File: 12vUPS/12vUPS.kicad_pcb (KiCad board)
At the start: 2 copper layers, 79 x 61 mm, 20 parts, among them J1 INPUT, J2 BATTERY, J3 OUTPUT, J4 ENABLE, K1 VEGHA L08A0212VDC, K2 VEGHA L08A0212VDC, Q1 BDX53C

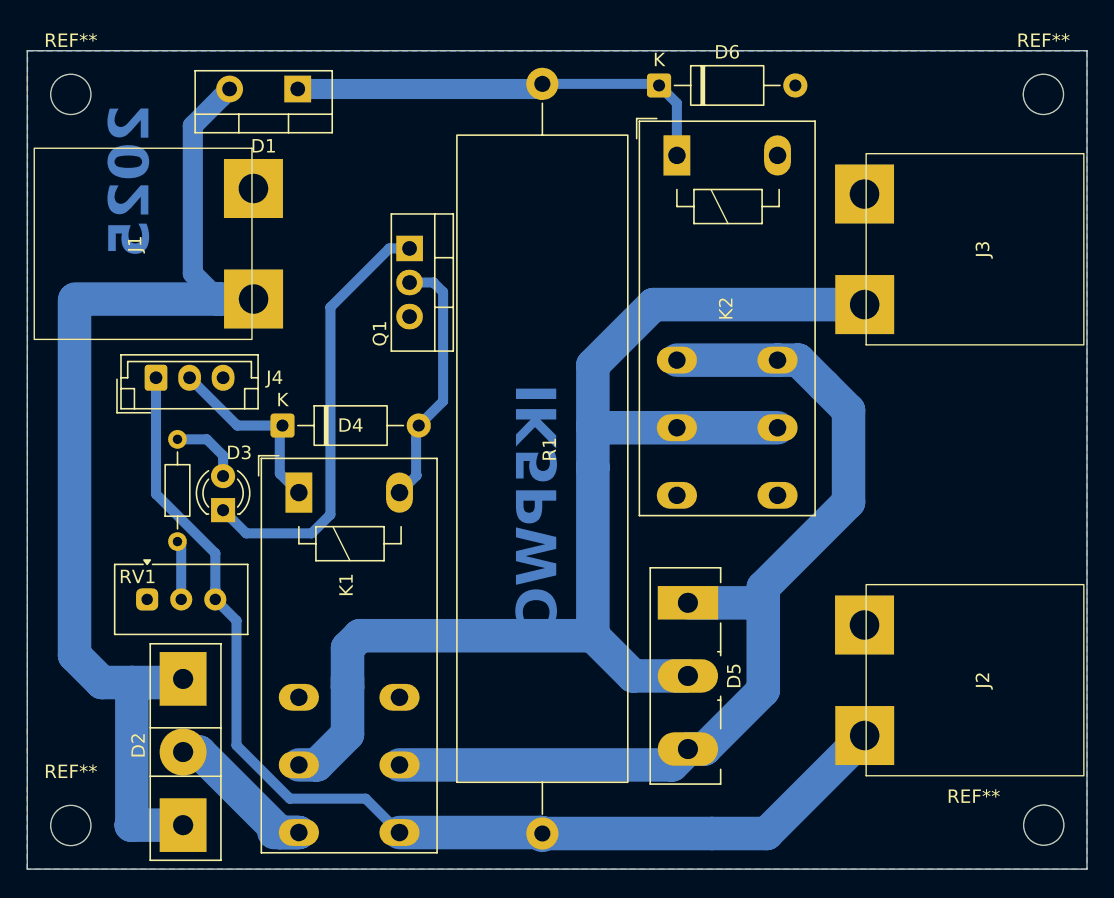
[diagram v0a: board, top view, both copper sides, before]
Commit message: Update 12vUPS-2025-06-10_185612.zip, 12vUPS-2025-06-10_190121.zip, 12vUPS-2025-06-10_190645.zip, and 3 more files
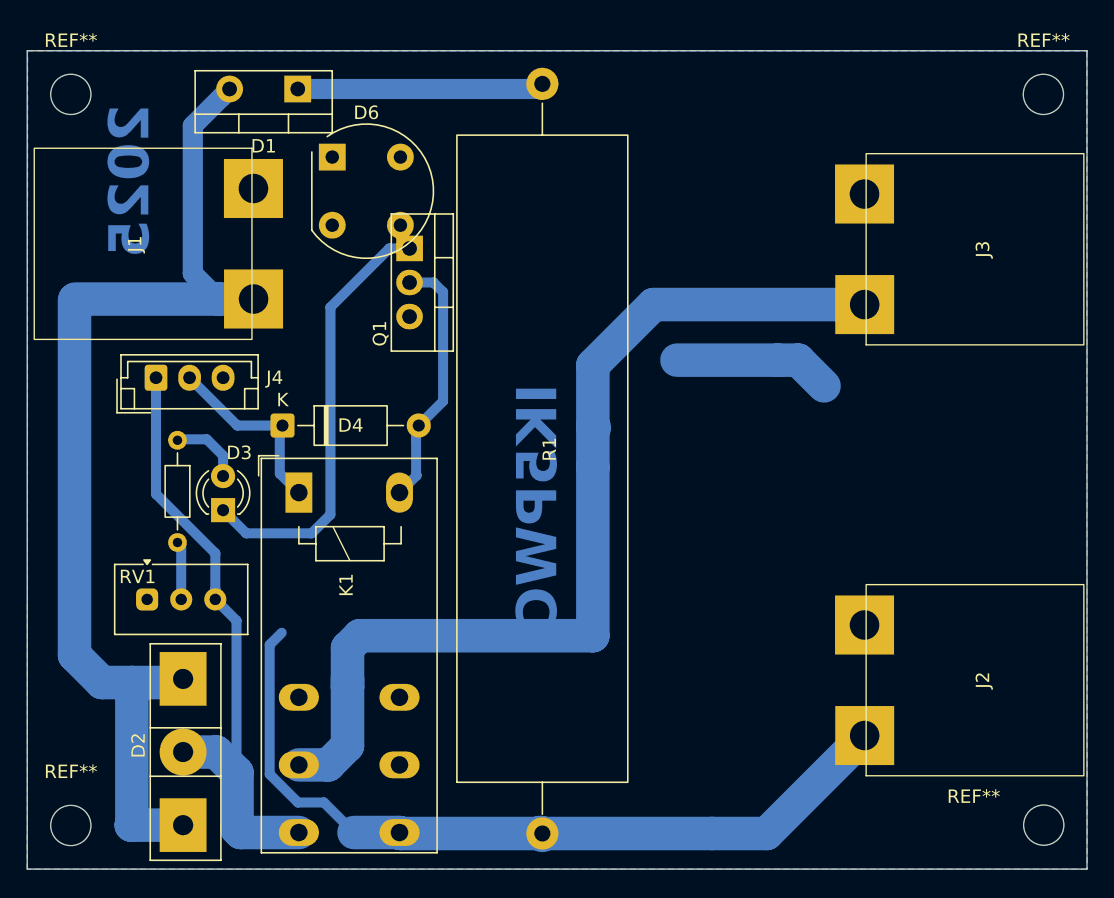
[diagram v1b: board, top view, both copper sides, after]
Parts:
- removed D5: D_Schottky_Dual_CommonCathode_AKA_Parallel, Package_TO_SOT_THT:TO-247-3_Vertical
- removed K2: VEGHA L08A0212VDC, IK5PWC:VEGhA L08 12V dc
- D6: value 1N4001 -> W01G; footprint Diode_THT:D_A-405_P10.16mm_Horizontal -> Diode_THT:Diode_Bridge_Round_D9.8mm
- moved D6 24.9 mm to (35.5, 24.3)
- moved R2 7.55 mm to (24.0, 45.4), turned to -90 degrees
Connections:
- D1 pad 1: /X1 -> Net-(D1-K)
- D1 pad 2: VCC -> /INPUT
- D2 pad 2: VCC -> /INPUT
- D6 pad 1: /X1 -> Net-(D6-+)
- D6 pad 2: GND -> /OUT
- J1 pad 2: VCC -> /INPUT
- J2 pad 1: /+12V -> /BATT
- J3 pad 1: Net-(D5-K) -> /OUT
- J4 pad 1: /+12V -> /BATT
- K1 pad 11: Net-(D5-K) -> /OUT
- K1 pad 24: /+12V -> /BATT
- R1 pad 1: /+12V -> /BATT
- R1 pad 2: /X1 -> Net-(D1-K)
- R2 pad 1: Net-(R2-Pad1) -> Net-(D3-A)
- R2 pad 2: Net-(D3-A) -> Net-(R2-Pad2)
- RV1 pad 2: Net-(R2-Pad1) -> Net-(R2-Pad2)
- RV1 pad 3: /+12V -> Net-(D6-+)
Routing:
- net Net-(D5-K): track 94.8 -> 0.00 mm
- net /OUT: track 0.00 -> 85.1 mm
- net /+12V: track 82.8 -> 0.00 mm
- net VCC: track 78.2 -> 0.00 mm
- net /INPUT: track 0.00 -> 78.2 mm
- net Net-(D7-A): track 72.9 -> 0.00 mm
- net /BATT: track 0.00 -> 60.5 mm
- net /X1: track 33.6 -> 0.00 mm
- net Net-(D2-K): track 13.0 -> 45.5 mm
- net Net-(D1-K): track 0.00 -> 19.1 mm
- net Net-(R2-Pad2): track 0.00 -> 4.43 mm
- net Net-(R2-Pad1): track 4.43 -> 0.00 mm

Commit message: Update #auto_saved_files#, 12vUPS-2025-06-02_175555.zip, 12vUPS-2025-06-02_180136.zip, and 18 more files
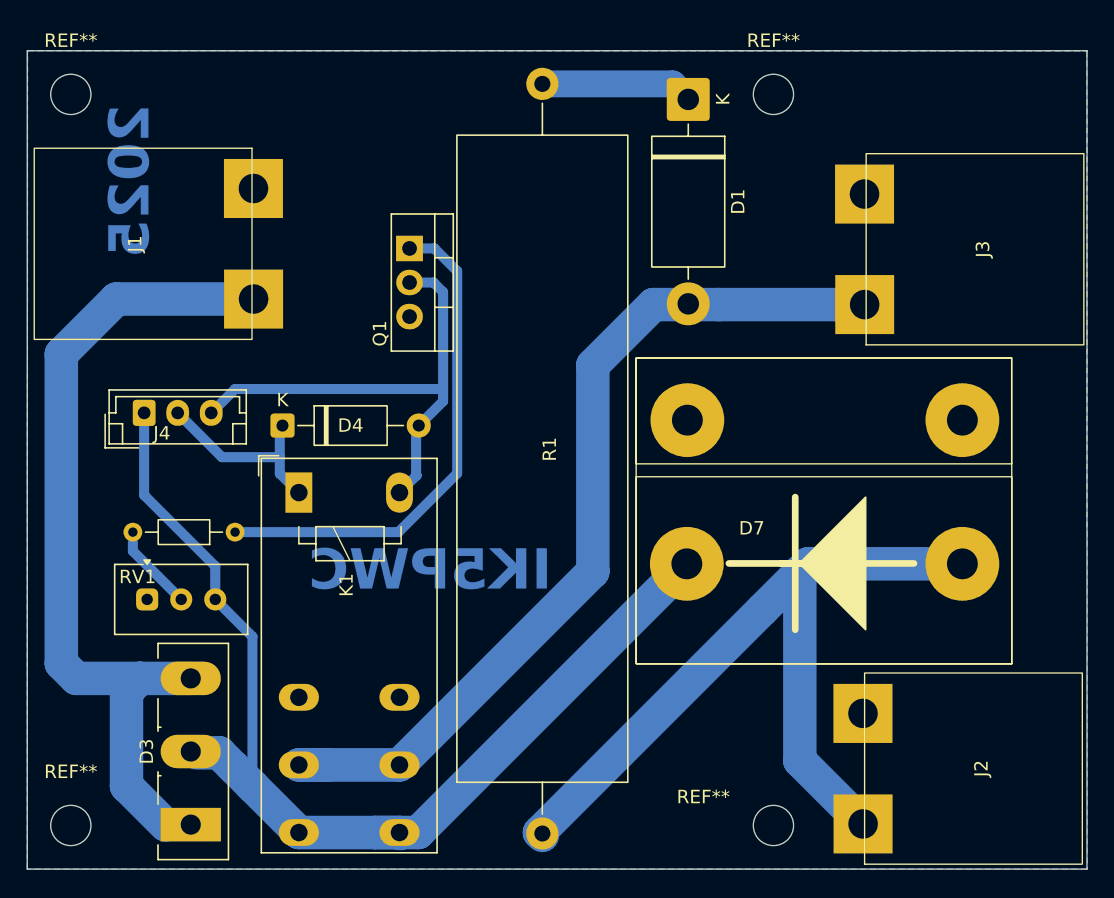
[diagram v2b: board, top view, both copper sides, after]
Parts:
- removed D2: 30CPF04, IK5PWC:30CPF04
- removed D6: W01G, Diode_THT:Diode_Bridge_Round_D9.8mm
- added D7: D_Ideal, IK5PWC:D_IDEAL_with_GND, F.Cu at (76.3, 58.9)
- D1: value BYW19 -> SF30GG; footprint Package_TO_SOT_THT:TO-220-2_Vertical -> Diode_THT:D_DO-201AD_P15.24mm_Horizontal
- D3: value LED_Small -> 60CPQ150; footprint LED_THT:LED_D3.0mm -> Package_TO_SOT_THT:TO-247-3_Vertical
- moved D1 29.1 mm to (62.1, 20.0), turned to -90 degrees
- moved D3 23.6 mm to (25.0, 74.1)
- moved REF** 20.1 mm to (68.4, 74.1)
- moved REF** 20.1 mm to (68.4, 19.6)
- moved R2 8.08 mm to (28.3, 52.3), turned to 180 degrees
- moved J2 6.59 mm to (75.1, 74.0)
- moved J4 2.76 mm to (21.5, 43.4)
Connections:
- D1 pad 2: /INPUT -> /OUT
- D3 pad 1: Net-(D3-K) -> /DC_IN
- D3 pad 2: Net-(D3-A) -> /DC-IN-RELE
- D4 pad 2: Net-(D4-A) -> /BJT-GND
- J1 pad 2: /INPUT -> /DC_IN
- J2 pad 1: /BATT -> /BATT_IN
- J4 pad 1: /BATT -> /DC-IN-RELE
- J4 pad 3: GND -> /BJT-GND
- K1 pad 14: Net-(D2-K) -> /DC-IN-RELE
- K1 pad 21: Net-(D7-A) -> /OUT
- K1 pad 24: /BATT -> /DC-IN-RELE
- K1 pad A2: Net-(D4-A) -> /BJT-GND
- Q1 pad 1: Net-(D3-K) -> Net-(Q1-B)
- Q1 pad 2: Net-(D4-A) -> /BJT-GND
- R1 pad 1: /BATT -> /BATT_IN
- R2 pad 1: Net-(D3-A) -> Net-(Q1-B)
- RV1 pad 3: Net-(D6-+) -> /DC-IN-RELE
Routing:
- net /DC-IN-RELE: track 0.00 -> 80.4 mm
- net /INPUT: track 78.2 -> 0.00 mm
- net /BATT_IN: track 0.00 -> 62.0 mm
- net /DC_IN: track 0.00 -> 61.8 mm
- net /BATT: track 60.5 -> 0.00 mm
- net Net-(D2-K): track 45.5 -> 0.00 mm
- net Net-(Q1-B): track 0.00 -> 37.7 mm
- net /BJT-GND: track 0.00 -> 37.5 mm
- net Net-(D3-K): track 32.5 -> 0.00 mm
- net Net-(D4-A): track 19.3 -> 0.00 mm
- net /OUT: track 85.1 -> 67.6 mm
- net Net-(D1-K): track 19.1 -> 12.2 mm
- net Net-(D3-A): track 5.43 -> 0.00 mm
- net Net-(R2-Pad2): track 4.43 -> 5.75 mm
- net /ENA: track 14.0 -> 14.5 mm

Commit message: Update 12vUPS-2025-06-06_224542.zip, 12vUPS-2025-06-06_225111.zip, 12vUPS-2025-06-06_225614.zip, and 28 more files
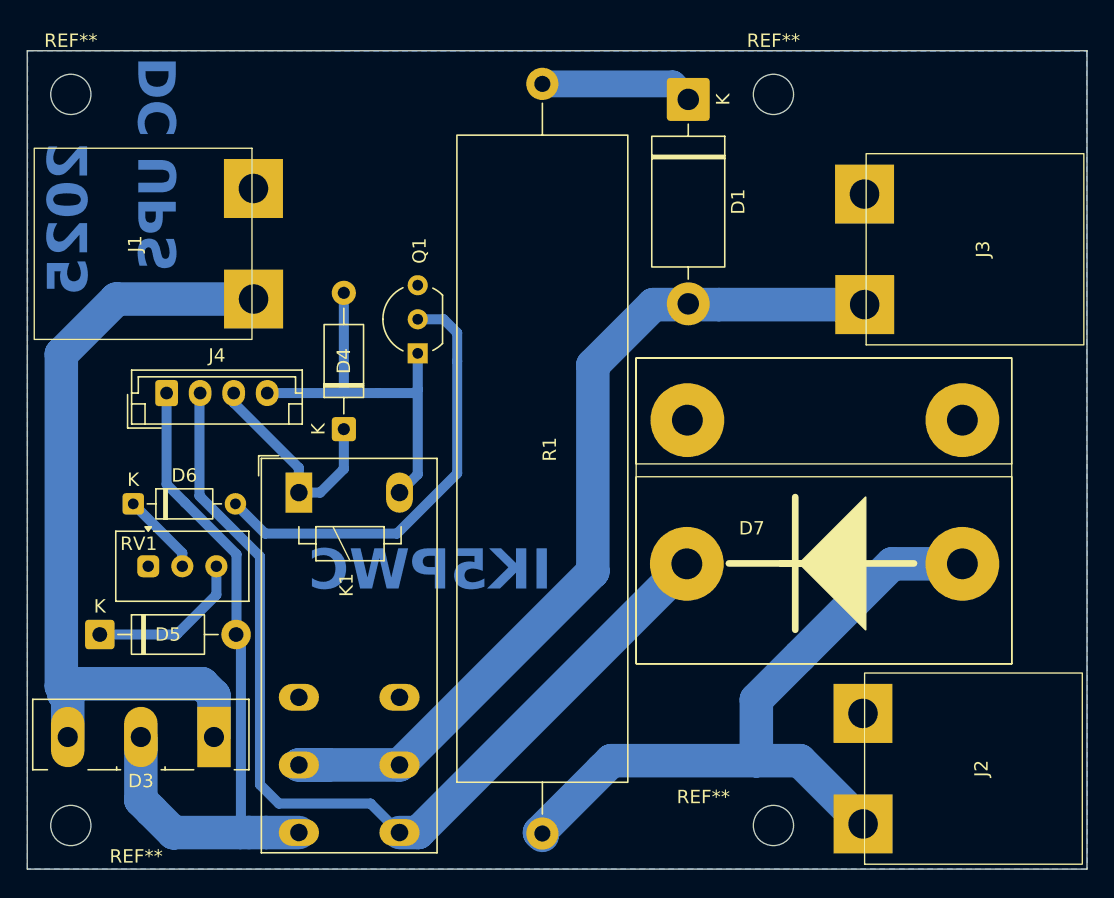
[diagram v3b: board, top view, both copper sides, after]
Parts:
- removed R2: 510, Resistor_THT:R_Axial_DIN0204_L3.6mm_D1.6mm_P7.62mm_Horizontal
- added D5: D, Diode_THT:D_DO-41_SOD81_P10.16mm_Horizontal, F.Cu at (18.2, 59.9)
- added D6: 4V1, Diode_THT:D_DO-35_SOD27_P7.62mm_Horizontal, F.Cu at (20.7, 50.2)
- J4: footprint Connector_JST:JST_EH_B3B-EH-A_1x03_P2.50mm_Vertical -> Connector_JST:JST_EH_B4B-EH-A_1x04_P2.50mm_Vertical
- Q1: value BDX53C -> BC337; footprint Package_TO_SOT_THT:TO-220-3_Vertical -> Package_TO_SOT_THT:TO-92_Inline_Wide
- moved Q1 7.84 mm to (41.9, 38.9), turned to 90 degrees
- moved D3 6.76 mm to (26.7, 67.5), turned to 180 degrees
- moved D4 4.58 mm to (36.4, 44.6), turned to 90 degrees
- moved RV1 2.47 mm to (21.8, 54.8)
- moved J4 2.23 mm to (23.2, 41.9)
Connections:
- D7 pad 1: /DC-IN-RELE -> Net-(D7-K)
- J4 pad 2: /ENA -> Net-(D7-K)
- J4 pad 3: /BJT-GND -> /ENA
- K1 pad 24: /DC-IN-RELE -> Net-(D7-K)
- Q1 pad 1: Net-(Q1-B) -> /BJT-GND
- Q1 pad 2: /BJT-GND -> Net-(D6-A)
- RV1 pad 3: /DC-IN-RELE -> Net-(D5-K)
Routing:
- net Net-(D7-K): track 0.00 -> 72.7 mm
- net Net-(Q1-B): track 37.7 -> 0.00 mm
- net Net-(D6-A): track 0.00 -> 33.1 mm
- net /DC-IN-RELE: track 80.4 -> 52.7 mm
- net Net-(D5-K): track 0.00 -> 12.0 mm
- net /BATT_IN: track 62.0 -> 53.8 mm
- net /BJT-GND: track 37.5 -> 29.8 mm
- net /DC_IN: track 61.8 -> 59.8 mm
- net /ENA: track 14.5 -> 16.5 mm
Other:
- board text added: "DC UPS"
